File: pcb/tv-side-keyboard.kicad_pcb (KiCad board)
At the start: 2 copper layers, 117 x 68 mm, 51 parts, among them J1 ESP-Prog-ProgramCOM-RECV, SW1 SW_Push, SW10 SW_Push, SW11 SW_Push, SW12 SW_Push, SW2 SW_Push, SW3 SW_Push, SW4 SW_Push, SW5 SW_Push, SW6 SW_Push, SW7 SW_Push, SW8 SW_Push, SW9 SW_Push, U1 M5StampS3, U2 M5 IR Unit

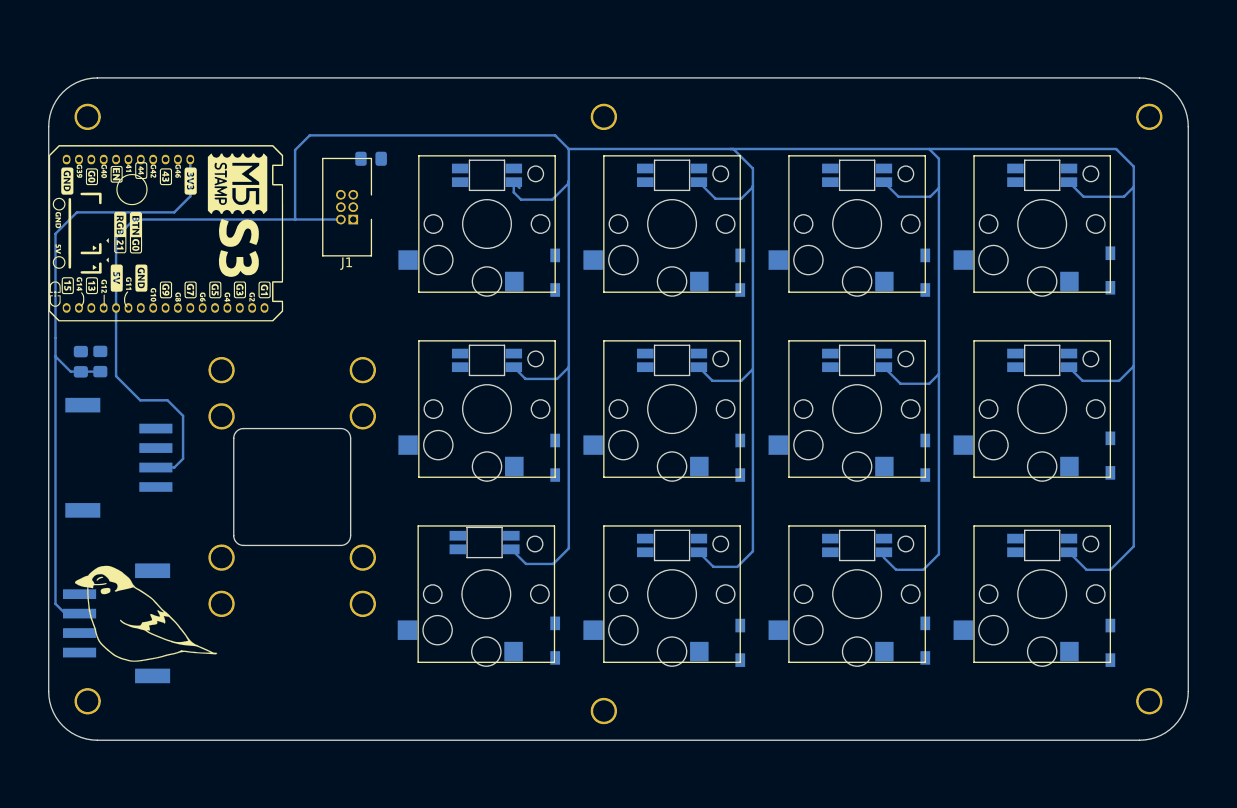
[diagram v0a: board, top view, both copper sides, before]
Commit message: build-pcb
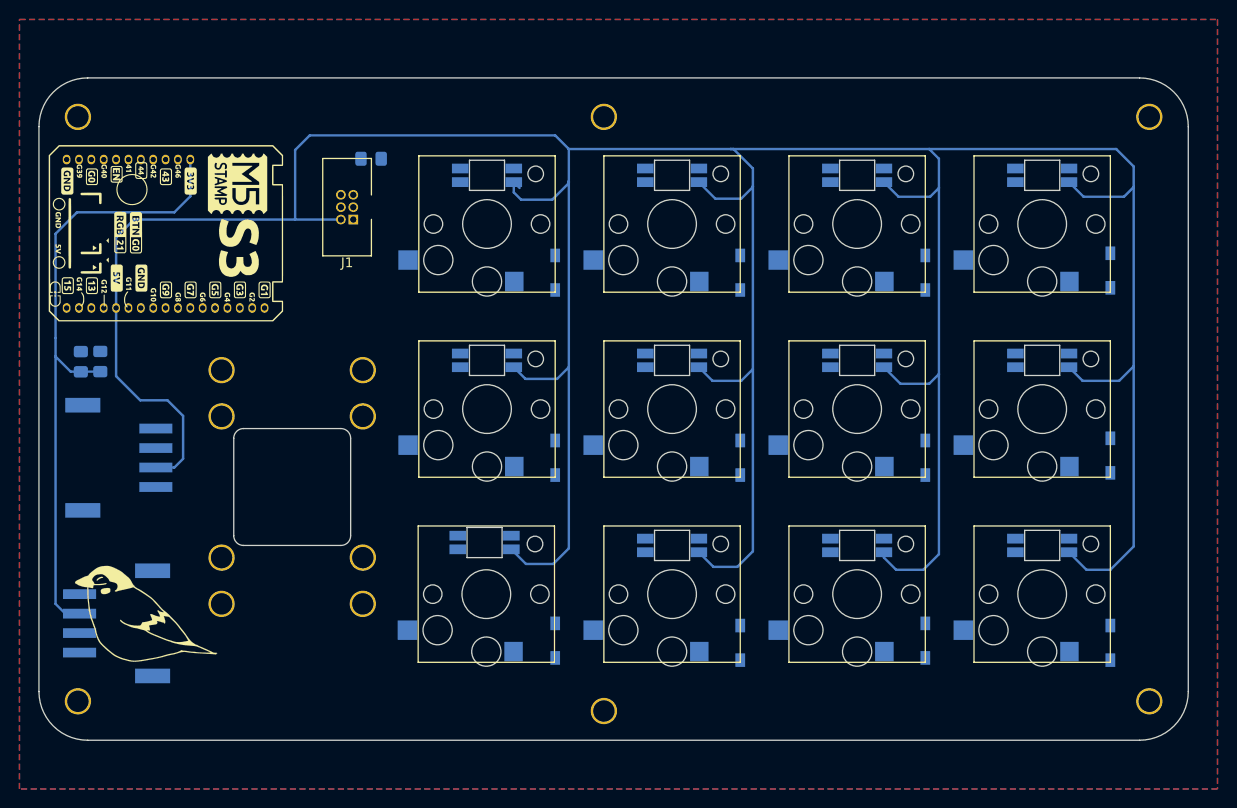
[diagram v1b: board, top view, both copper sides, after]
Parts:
- moved H2 1.00 mm to (57.0, 34.0)
- moved H7 1.00 mm to (57.0, 94.0)
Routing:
- added copper zone on B.Cu, net GND
- added copper zone on F.Cu, net GND
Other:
- board size 117 x 68 mm -> 118 x 68 mm
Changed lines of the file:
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@@
   )
   (footprint "$sparrow62:M2_v2" (layer "F.Cu")
-    (at 58 94)
+    (at 57 94)
     (attr through_hole)
     (fp_text reference "H7" (at 0 1.905) (layer "Dwgs.User") hide
@@
   )
   (footprint "$sparrow62:M2_v2" (layer "F.Cu")
-    (at 58 34)
+    (at 57 34)
     (attr through_hole)
     (fp_text reference "H2" (at 0 1.905) (layer "Dwgs.User") hide
@@
   (gr_arc (start 171 93) (mid 169.535534 96.535534) (end 166 98)
     (stroke (width 0.1) (type default)) (layer "Edge.Cuts"))
-  (gr_arc (start 54 35) (mid 55.464466 31.464466) (end 59 30)
+  (gr_arc (start 53 35) (mid 54.464466 31.464466) (end 58 30)
     (stroke (width 0.1) (type default)) (layer "Edge.Cuts"))
-  (gr_arc (start 59 98) (mid 55.464466 96.535534) (end 54 93)
+  (gr_arc (start 58 98) (mid 54.464466 96.535534) (end 53 93)
     (stroke (width 0.1) (type default)) (layer "Edge.Cuts"))
-  (gr_line (start 59 30) (end 166 30)
+  (gr_line (start 58 30) (end 166 30)
     (stroke (width 0.1) (type default)) (layer "Edge.Cuts"))
-  (gr_line (start 54 93) (end 54 35)
+  (gr_line (start 53 93) (end 53 35)
     (stroke (width 0.1) (type default)) (layer "Edge.Cuts"))
   (gr_arc (start 166 30) (mid 169.535534 31.464466) (end 171 35)
     (stroke (width 0.1) (type default)) (layer "Edge.Cuts"))
-  (gr_line (start 166 98) (end 59 98)
+  (gr_line (start 166 98) (end 58 98)
     (stroke (width 0.1) (type default)) (layer "Edge.Cuts"))
   (gr_line (start 171 35) (end 171 93)
@@
   (segment (start 106.2 60.9) (end 107.4 59.7) (width 0.25) (layer "B.Cu") (net 15))
   (segment (start 103 79.9) (end 101.5 78.4) (width 0.25) (layer "B.Cu") (net 15))
+  (zone (net 4) (net_name "GND") (layers "F&B.Cu") (hatch edge 0.5)
+    (connect_pads (clearance 0.5))
+    (min_thickness 0.25) (filled_areas_thickness no)
+    (fill yes (thermal_gap 0.5) (thermal_bridge_width 0.5))
+    (polygon
+      (pts
+        (xy 51 24)
+        (xy 174 24)
+        (xy 174 103)
+        (xy 51 103)
+      )
+    )
+  )
 )
